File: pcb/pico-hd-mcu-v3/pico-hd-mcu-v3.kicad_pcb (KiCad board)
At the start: 2 copper layers, 87.9 x 88 mm, 53 parts

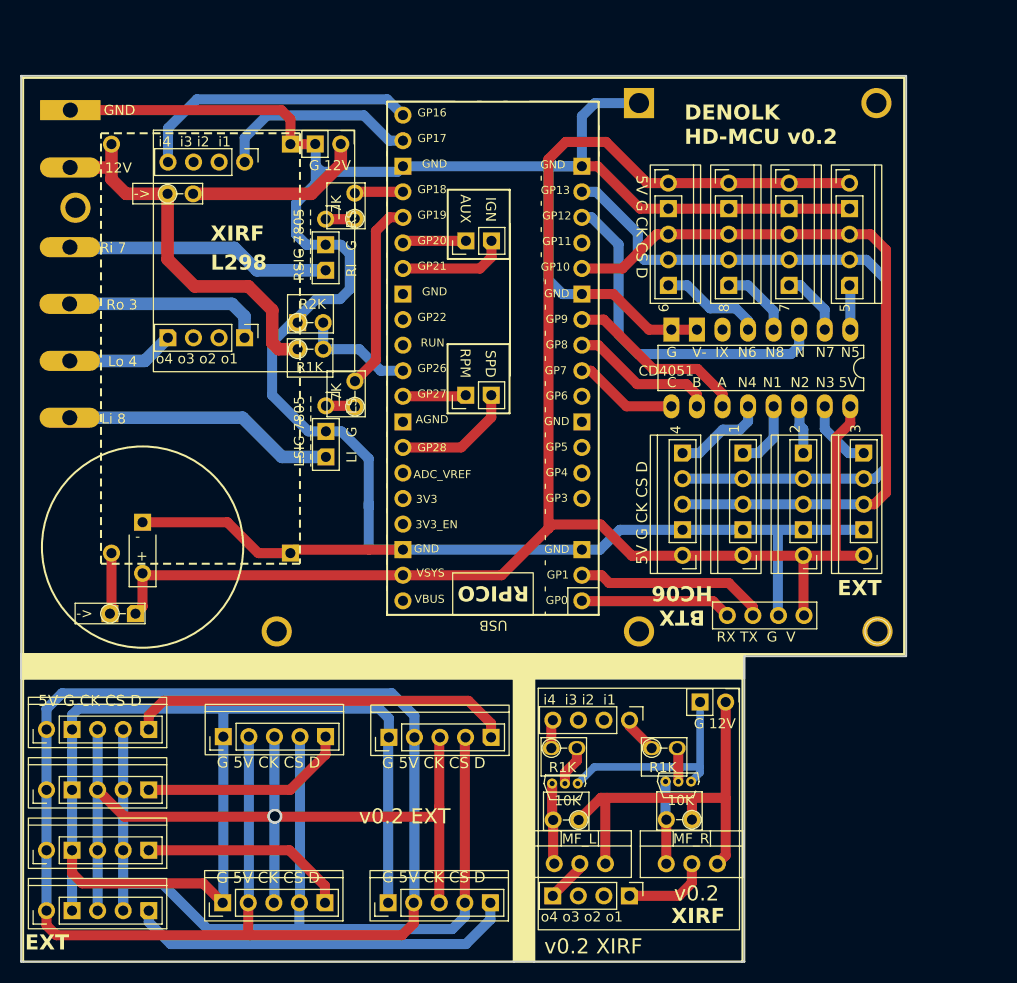
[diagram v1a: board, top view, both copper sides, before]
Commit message: pcbv3 stub
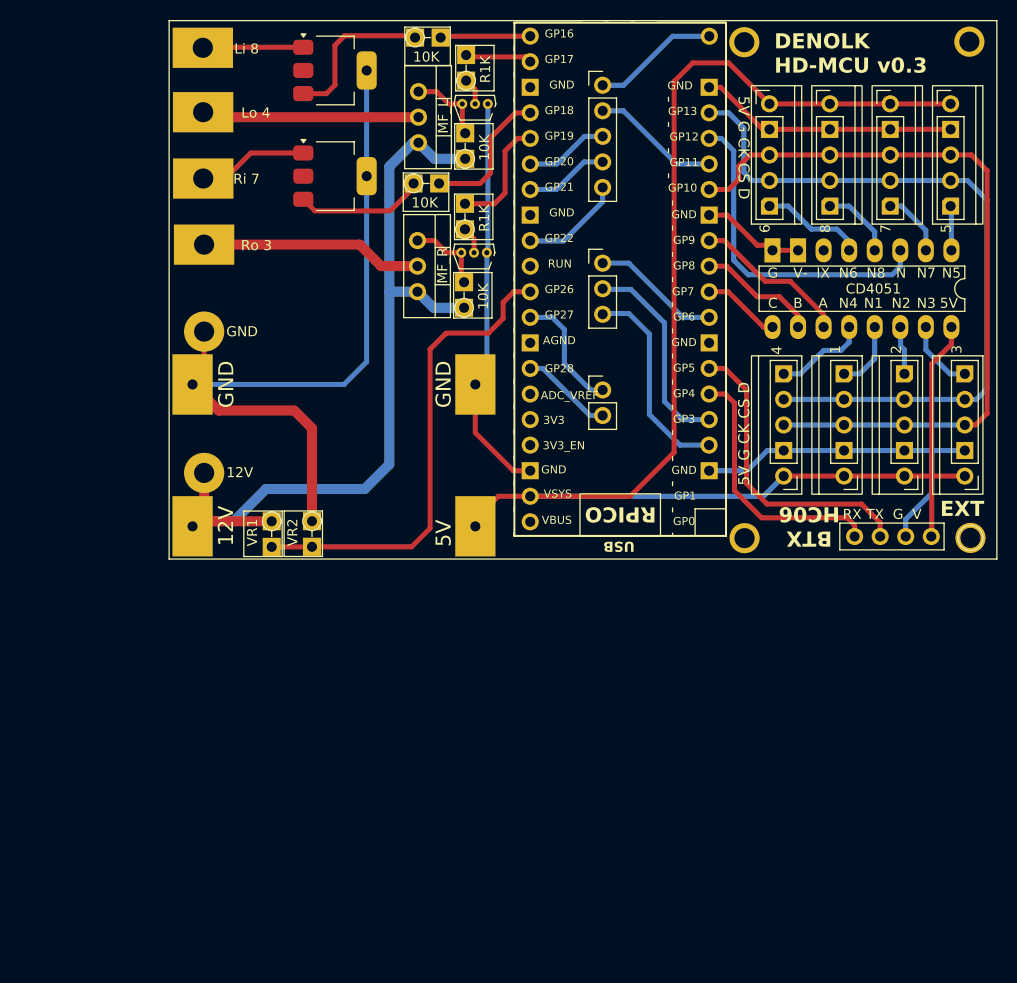
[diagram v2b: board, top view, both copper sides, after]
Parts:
- removed -> (x2), 7K (x2), R2K: R_Axial_DIN0204_L3.6mm_D1.6mm_P2.54mm_Vertical, Resistor_THT:R_Axial_DIN0204_L3.6mm_D1.6mm_P2.54mm_Vertical
- removed the 1 at (24.3, 97.5)
- removed the 1 at (41.9, 92.2)
- removed the 10K at (77.2, 100.5)
- removed the 10K at (88.5, 100.5)
- removed the 2 at (24.3, 103.5)
- removed the 2 at (41.8, 108.8)
- removed the 3 at (58.3, 108.8)
- removed the 3 at (24.3, 109.5)
- removed the 4 at (58.4, 92.3)
- removed the 4 at (24.3, 91.5)
- removed the ? at (27.2, 39.7)
- removed the ? at (26.7, 30.0)
- removed the ? at (47.1, 81.8)
- removed the ? at (26.7, 35.7)
- removed LSIG 7805: PinSocket_1x03_P2.54mm_Vertical, Connector_PinSocket_2.54mm:PinSocket_1x03_P2.54mm_Vertical
- removed the R1K at (74.5, 93.4)
- removed the R1K at (49.3, 53.8)
- removed the R1K at (84.5, 93.4)
- removed the REF** at (88.4, 96.7)
- removed the REF** at (66.0, 43.0)
- removed the REF** at (85.9, 104.9)
- removed the REF** at (39.7, 58.2)
- removed the REF** at (74.8, 104.9)
- removed the REF** at (83.2, 97.9)
- removed the REF** at (45.0, 42.5)
- removed the REF** at (77.1, 96.9)
- removed the REF** at (33.9, 73.2)
- removed the REF** at (66.0, 58.3)
- removed RSIG 7805: PinSocket_1x03_P2.54mm_Vertical, Connector_PinSocket_2.54mm:PinSocket_1x03_P2.54mm_Vertical
- added 10K: R_Axial_DIN0204_L3.6mm_D1.6mm_P2.54mm_Vertical, Resistor_THT:R_Axial_DIN0204_L3.6mm_D1.6mm_P2.54mm_Vertical, F.Cu at (61.0, 22.8)
- added 10K: R_Axial_DIN0204_L3.6mm_D1.6mm_P2.54mm_Vertical, Resistor_THT:R_Axial_DIN0204_L3.6mm_D1.6mm_P2.54mm_Vertical, F.Cu at (65.8, 49.6)
- added 10K: R_Axial_DIN0204_L3.6mm_D1.6mm_P2.54mm_Vertical, Resistor_THT:R_Axial_DIN0204_L3.6mm_D1.6mm_P2.54mm_Vertical, F.Cu at (60.8, 37.3)
- added 10K: R_Axial_DIN0204_L3.6mm_D1.6mm_P2.54mm_Vertical, Resistor_THT:R_Axial_DIN0204_L3.6mm_D1.6mm_P2.54mm_Vertical, F.Cu at (65.9, 34.8)
- added ?: , , F.Cu at (90.2, 22.6)
- added ?: , , F.Cu at (40.0, 52.0)
- added ?: , , F.Cu at (90.2, 63.3)
- added ?: , , F.Cu at (40.0, 66.0)
- added R1K: R_Axial_DIN0204_L3.6mm_D1.6mm_P2.54mm_Vertical, Resistor_THT:R_Axial_DIN0204_L3.6mm_D1.6mm_P2.54mm_Vertical, F.Cu at (65.9, 41.8)
- added R1K: R_Axial_DIN0204_L3.6mm_D1.6mm_P2.54mm_Vertical, Resistor_THT:R_Axial_DIN0204_L3.6mm_D1.6mm_P2.54mm_Vertical, F.Cu at (66.0, 27.1)
- added REF**: MF_L, Package_TO_SOT_THT:TO-220-3_Vertical, F.Cu at (61.3, 28.2)
- added REF**: PinHeader_1x05_P2.54mm_Vertical, Connector_PinHeader_2.54mm:PinHeader_1x05_P2.54mm_Vertical, F.Cu at (79.6, 27.5)
- added REF**: PinHeader_1x03_P2.54mm_Vertical, Connector_PinHeader_2.54mm:PinHeader_1x03_P2.54mm_Vertical, F.Cu at (79.6, 45.2)
- added REF**: P12V5, footprints:P12V5, B.Cu at (36.9, 54.3)
- added REF**: RS78, Package_TO_SOT_SMD:SOT-223, F.Cu at (53.0, 36.6)
- added REF**: 22RG, Package_TO_SOT_THT:TO-92S, F.Cu at (68.1, 44.2)
- added REF**: LS78, Package_TO_SOT_SMD:SOT-223, F.Cu at (53.0, 26.1)
- added REF**: MF_R, Package_TO_SOT_THT:TO-220-3_Vertical, F.Cu at (61.2, 43.0)
- added REF**: PinHeader_1x02_P2.54mm_Vertical, Connector_PinHeader_2.54mm:PinHeader_1x02_P2.54mm_Vertical, F.Cu at (79.6, 57.8)
- added REF**: 22LF, Package_TO_SOT_THT:TO-92S, F.Cu at (68.2, 29.4)
- added VR1: R_Axial_DIN0204_L3.6mm_D1.6mm_P2.54mm_Vertical, Resistor_THT:R_Axial_DIN0204_L3.6mm_D1.6mm_P2.54mm_Vertical, F.Cu at (46.7, 70.9)
- added VR2: R_Axial_DIN0204_L3.6mm_D1.6mm_P2.54mm_Vertical, Resistor_THT:R_Axial_DIN0204_L3.6mm_D1.6mm_P2.54mm_Vertical, F.Cu at (50.7, 70.8)
- moved ? 39.1 mm to (39.8, 23.8)
- moved ? 28.0 mm to (39.9, 30.2), turned to 180 degrees
- moved ? 14.9 mm to (39.9, 36.8)
- moved REF** 14.9 mm to (81.3, 46.1)
- moved ? 14.9 mm to (103.1, 73.7)
- moved ? 14.6 mm to (40.0, 43.4)
- moved ? 14.0 mm to (93.7, 72.5)
- moved REF** 13.1 mm to (116.2, 72.5)
- moved 1 12.8 mm to (103.6, 66.4)
- moved 2 12.8 mm to (109.6, 66.4)
- moved 3 12.8 mm to (115.6, 66.4)
- moved 4 12.8 mm to (97.6, 66.4)
- moved 5 12.8 mm to (114.2, 29.4)
- moved 6 12.8 mm to (96.2, 29.4)
- moved 7 12.8 mm to (108.2, 29.4)
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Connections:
- ? pad 1: GND -> (no net)
- REF** pad 15: (no net) -> AUX_G11
- REF** pad 21: D_SIG_L_OUT -> D_SIG_L_IN
- REF** pad 22: D_SIG_R_OUT -> D_SIG_L_OUT
- REF** pad 23: GND -> (no net)
- REF** pad 25: D_SIG_L_IN -> D_SIG_R_OUT
- REF** pad 26: D_AUX -> AUX_G20
- REF** pad 27: D_IGN -> AUX_G21
- REF** pad 29: (no net) -> AUX_G22
- REF** pad 32: D_RPM -> AUX_A1
- REF** pad 34: D_SPD -> AUX_A2
- REF** pad 5: (no net) -> AUX_G3
- REF** pad 6: (no net) -> D_BT_TX
- REF** pad 7: (no net) -> D_BT_RX
- REF** pad 9: (no net) -> AUX_G6
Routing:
- net x5V: track 137.6 -> 0.00 mm
- net xGND: track 107.8 -> 0.00 mm
- net xD_CS: track 92.5 -> 0.00 mm
- net (no net): track 104.8 -> 15.4 mm
- net xD_SCK: track 86.1 -> 0.00 mm, vias 1 -> 0
- net GND: track 270.8 -> 190.7 mm
- net xMUX_S3: track 38.7 -> 0.00 mm
- net xMUX_S4: track 38.3 -> 0.00 mm
- net D_VOLT: track 11.5 -> 47.6 mm
- net 12V: track 56.8 -> 82.9 mm
- net xMUX_S1: track 20.8 -> 0.00 mm
- net AUX_G2: track 0.00 -> 20.7 mm
- net xMUX_S2: track 20.7 -> 0.00 mm
- net AUX_G3: track 0.00 -> 20.5 mm
- net 5V: track 176.0 -> 155.7 mm
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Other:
- board outline removed
- board text added: "5V"
- board text added: "AUX_G11"
- board text added: "AUX_G15"
- board text added: "AUX_G2"
- board text added: "AUX_G20"
- board text added: "AUX_G21"
- board text added: "AUX_G22"
- board text added: "AUX_G27 A1"
- board text added: "AUX_G28 A2"
- board text added: "AUX_G3"
- board text added: "AUX_G6"
- board text added: "DENOLK HD-MCU v0.3"
- board text removed: "12V REG"
- board text removed: "AUX"
- board text removed: "DENOLK HD-MCU v0.2"
- board text removed: "G 5V CK CS D"
- board text removed: "IGN"
- board text removed: "RPM"
- board text removed: "SPD"
- board text removed: "XIRF"
- board text removed: "v0.2"
- board text removed: "v0.2 EXT"
- board text removed: "v0.2 XIRF"
